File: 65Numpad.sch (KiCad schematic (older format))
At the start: 137 parts, among them J1 MX-NoLED, K1 MX-NoLED, M1 MX-NoLED, P1 MX-NoLED, Q1 MX-NoLED, T1 MX-NoLED, U1 ProMicro, U2 MX-NoLED, X1 MX-NoLED, Y1 MX-NoLED

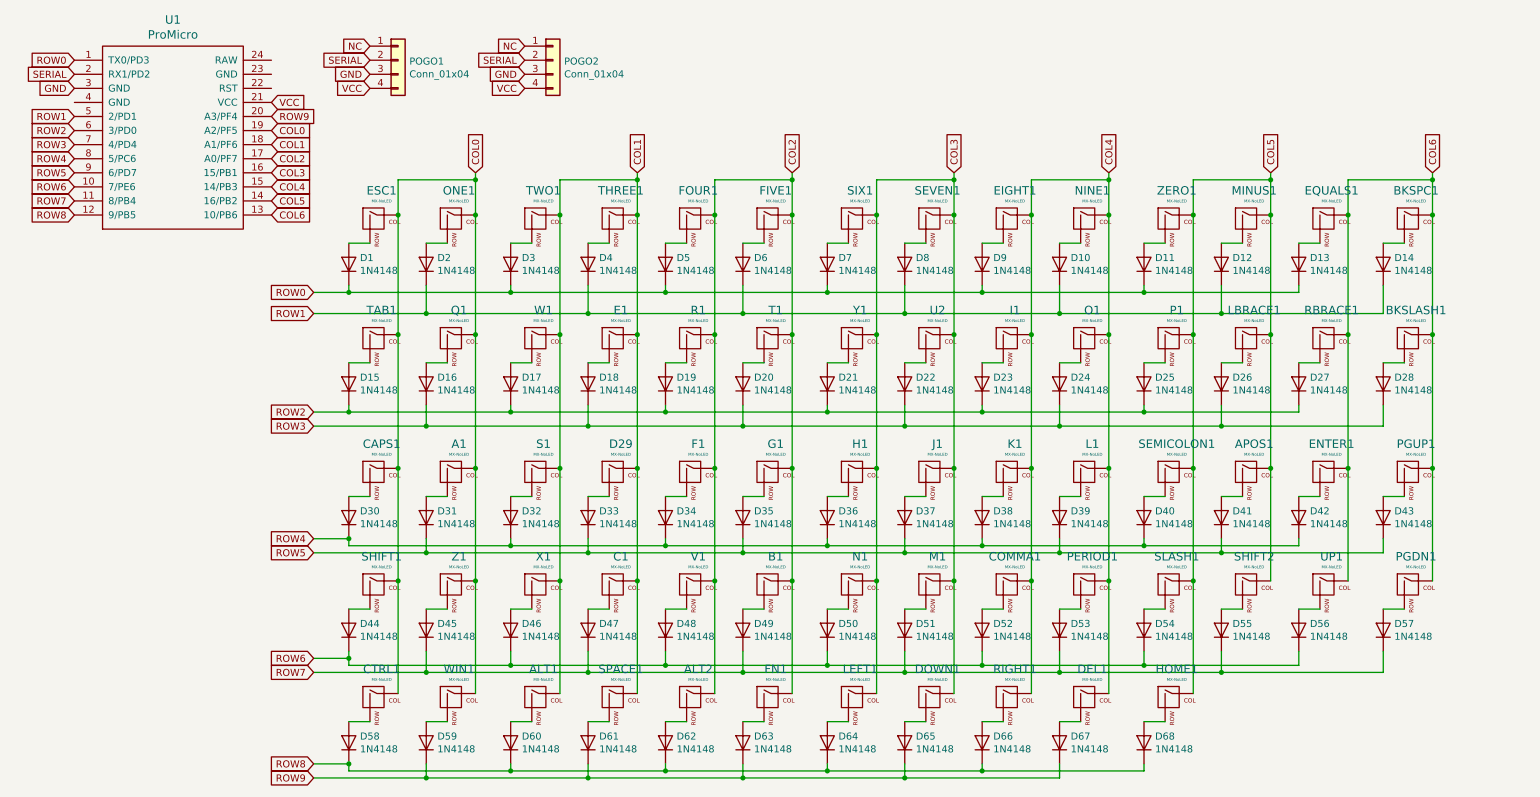
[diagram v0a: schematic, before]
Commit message: Arranged PCB
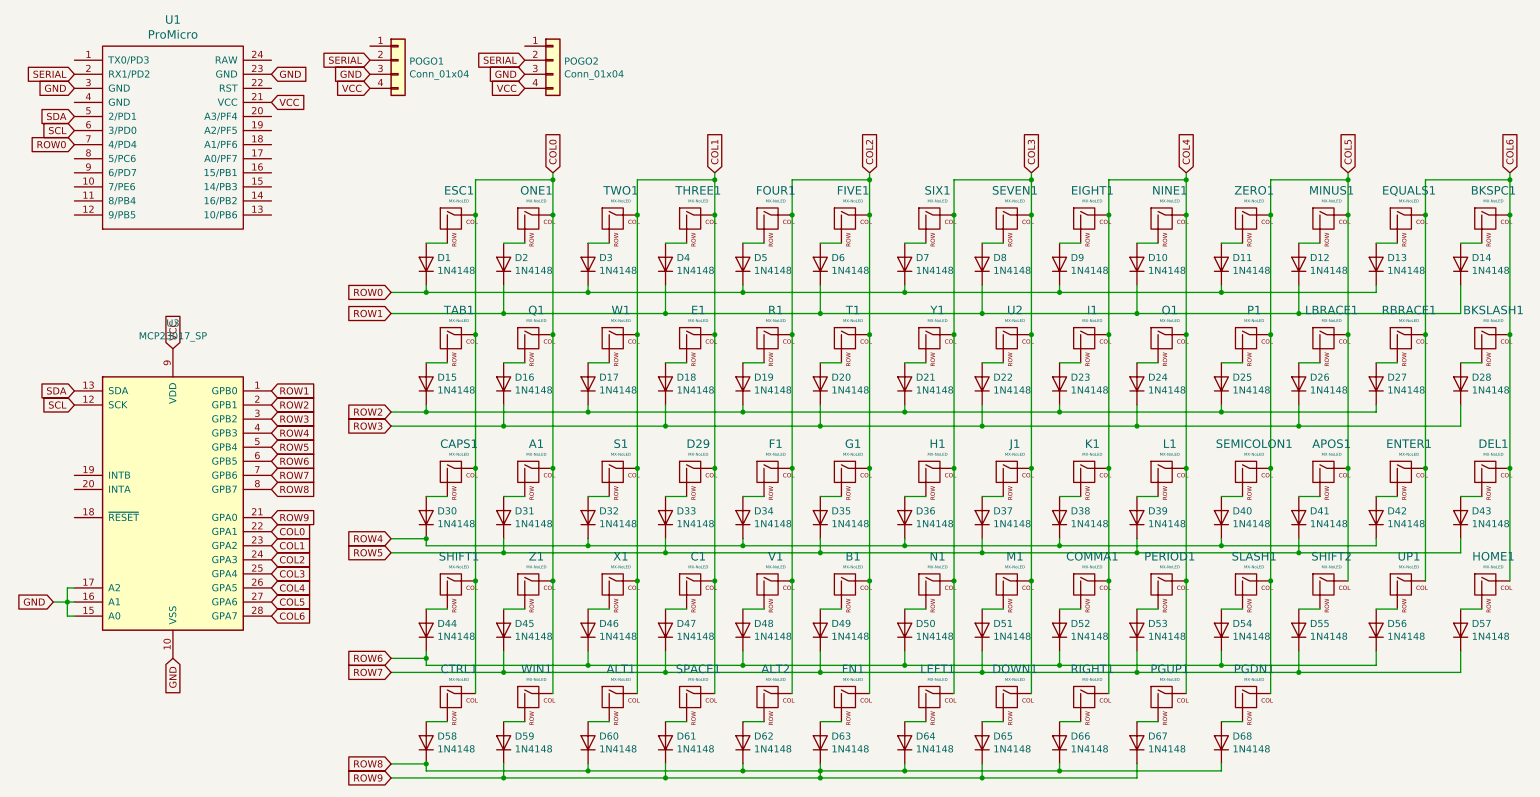
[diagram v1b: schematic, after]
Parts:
- added U3: MCP23017_SP, Package_DIP:DIP-28_W7.62mm, symbol Interface_Expansion:MCP23017_SP
- A1, APOS1, B1, C1, COMMA1, D29, DEL1, DOWN1, E1, EIGHT1, EQUALS1, ESC1, F1, FIVE1, FOUR1, G1, H1, HOME1, I1, J1, K1, L1, LBRACE1, LEFT1, M1, MINUS1, N1, NINE1, O1, ONE1, P1, PERIOD1, PGDN1, PGUP1, Q1, R1, RBRACE1, RIGHT1, S1, SEMICOLON1, SEVEN1, SIX1, SLASH1, T1, THREE1, TWO1, U2, UP1, V1, W1, X1, Y1, Z1, ZERO1: footprint MX_Only:MXOnly-1U-NoLED -> MX_Only:MXOnly-1U-NoLEDHotswap
- ALT1, ALT2, CTRL1, FN1, WIN1: footprint MX_Only:MXOnly-1.25U-NoLED -> MX_Only:MXOnly-1.25U-NoLEDHotswap
- BKSLASH1, TAB1: footprint MX_Only:MXOnly-1.5U-NoLED -> MX_Only:MXOnly-1.5U-NoLEDHotswap
- BKSPC1: footprint MX_Only:MXOnly-2U-NoLED -> MX_Only:MXOnly-2U-NoLEDHotswap
- CAPS1, SHIFT2: footprint MX_Only:MXOnly-1.75U-NoLED -> MX_Only:MXOnly-1.75U-NoLEDHotswap
- D1, D10, D11, D12, D13, D14, D15, D16, D17, D18, D19, D2, D20, D21, D22, D23, D24, D25, D26, D27, D28, D3, D30, D31, D32, D33, D34, D35, D36, D37, D38, D39, D4, D40, D41, D42, D43, D44, D45, D46, D47, D48, D49, D5, D50, D51, D52, D53, D54, D55, D56, D57, D58, D59, D6, D60, D61, D62, D63, D64, D65, D66, D67, D68, D7, D8, D9: footprint Diode_THT:D_DO-35_SOD27_P7.62mm_Horizontal -> Diodes_THT:D_DO-35_SOD27_P7.62mm_Horizontal
- ENTER1, SHIFT1: footprint MX_Only:MXOnly-2.25U-NoLED -> MX_Only:MXOnly-2.25U-NoLEDHotswap
- SPACE1: footprint MX_Only:MXOnly-6.25U-NoLED -> MX_Only:MXOnly-6.25U-NoLEDHotswap
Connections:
- net COL0: now also U3.22 (GPA1); no longer U1.19 (A2/PF5)
- net COL1: now also U3.23 (GPA2); no longer U1.18 (A1/PF6)
- net COL2: now also U3.24 (GPA3); no longer U1.17 (A0/PF7)
- net COL3: now also U3.25 (GPA4); no longer U1.16 (15/PB1)
- net COL4: now also PGUP1.1 (COL), U3.26 (GPA5); no longer DEL1.1 (COL), U1.15 (14/PB3)
- net COL5: now also PGDN1.1 (COL), U3.27 (GPA6); no longer HOME1.1 (COL), U1.14 (16/PB2)
- net COL6: now also DEL1.1 (COL), HOME1.1 (COL), U3.28 (GPA7); no longer PGDN1.1 (COL), PGUP1.1 (COL), U1.13 (10/PB6)
- net GND: now also U1.23 (GND), U3.10 (VSS), U3.15 (A0), U3.16 (A1), U3.17 (A2)
- net ROW0: now also U1.7 (4/PD4); no longer U1.1 (TX0/PD3)
- net ROW1: now also U3.1 (GPB0); no longer U1.5 (2/PD1)
- net ROW2: now also U3.2 (GPB1); no longer U1.6 (3/PD0)
- net ROW3: now also U3.3 (GPB2); no longer U1.7 (4/PD4)
- net ROW4: now also U3.4 (GPB3); no longer U1.8 (5/PC6)
- net ROW5: now also U3.5 (GPB4); no longer U1.9 (6/PD7)
- net ROW6: now also U3.6 (GPB5); no longer U1.10 (7/PE6)
- net ROW7: now also U3.7 (GPB6); no longer U1.11 (8/PB4)
- net ROW8: now also D59.1 (K), D61.1 (K), D63.1 (K), D65.1 (K), D67.1 (K), U3.21 (GPA0), U3.8 (GPB7); no longer U1.12 (9/PB5)
- net VCC: now also U3.9 (VDD)
- net at DEL1.2 (ROW): now also D43.2 (A); no longer D67.2 (A)
- net at HOME1.2 (ROW): now also D57.2 (A); no longer D68.2 (A)
- net at PGUP1.2 (ROW): now also D67.2 (A); no longer D43.2 (A)
- net at PGDN1.2 (ROW): now also D68.2 (A); no longer D57.2 (A)
- net NC: no longer names the net of POGO2.1 (Pin_1)
- net NC: no longer POGO1.1 (Pin_1)
- removed net ROW9: D59.1 (K), D61.1 (K), D63.1 (K), D65.1 (K), D67.1 (K), U1.20 (A3/PF4)
- new net SCL: U1.6 (3/PD0), U3.12 (SCK)
- new net SDA: U1.5 (2/PD1), U3.13 (SDA)
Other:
- moved on the sheet: A1, ALT1, ALT2, APOS1, B1, BKSLASH1, BKSPC1, C1, CAPS1, COMMA1, CTRL1, D1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

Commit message: Almost done routing
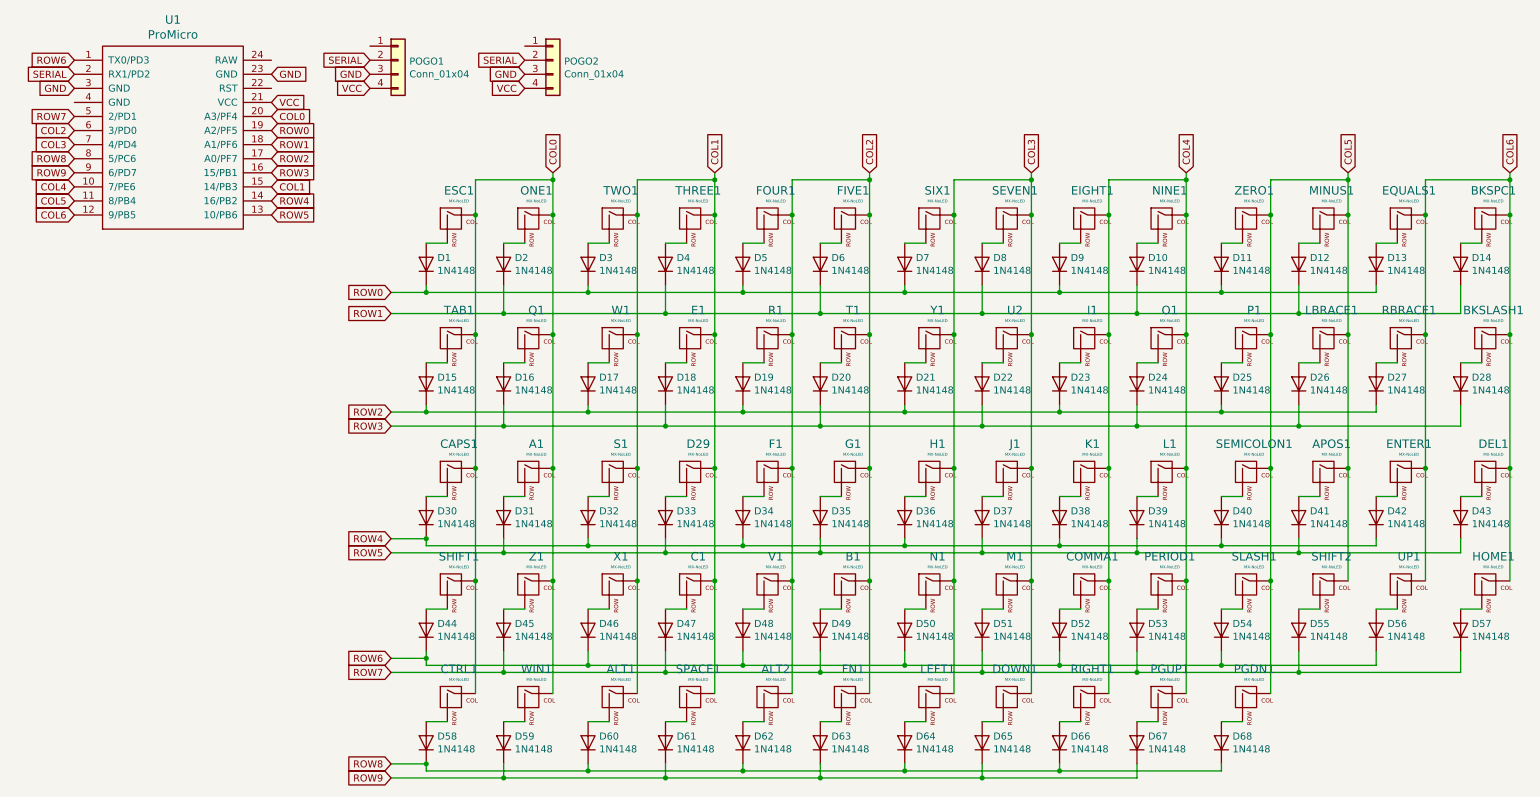
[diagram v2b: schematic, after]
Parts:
- removed U3: MCP23017_SP, Package_DIP:DIP-28_W7.62mm, symbol Interface_Expansion:MCP23017_SP
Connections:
- net SCL is gone; now on net COL2: U1.6 (3/PD0)
- net SDA is gone; now on net ROW7: U1.5 (2/PD1)
- net COL0: now also U1.20 (A3/PF4)
- net COL1: now also U1.15 (14/PB3)
- net COL3: now also U1.7 (4/PD4)
- net COL4: now also U1.10 (7/PE6)
- net COL5: now also U1.11 (8/PB4)
- net COL6: now also U1.12 (9/PB5)
- net ROW0: now also U1.19 (A2/PF5); no longer U1.7 (4/PD4)
- net ROW1: now also U1.18 (A1/PF6)
- net ROW2: now also U1.17 (A0/PF7)
- net ROW3: now also U1.16 (15/PB1)
- net ROW4: now also U1.14 (16/PB2)
- net ROW5: now also U1.13 (10/PB6)
- net ROW6: now also U1.1 (TX0/PD3)
- net ROW8: now also U1.8 (5/PC6); no longer D59.1 (K), D61.1 (K), D63.1 (K), D65.1 (K), D67.1 (K)
- net ROW9: now reaches U1.9 (6/PD7)
- net ROW9: now also D59.1 (K), D61.1 (K), D63.1 (K), D65.1 (K), D67.1 (K)
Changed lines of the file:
@@
 Connection ~ 3350 6000
-Wire Wire Line
-	6150 6050 6750 6050
 Wire Wire Line
 	3900 6000 3900 6100
@@
 	5600 6000 5600 6050
 Connection ~ 5600 6050
-Wire Wire Line
-	5600 6050 6150 6050
 Connection ~ 6150 6100
 Wire Wire Line
@@
 Text GLabel 4050 1100 0    50   Input ~ 0
 GND
-$Comp
-L Interface_Expansion:MCP23017_SP U3
-U 1 1 602098ED
-P 1550 4150
-F 0 "U3" H 1550 5431 50  0000 C CNN
-F 1 "MCP23017_SP" H 1550 5340 50  0000 C CNN
-F 2 "Package_DIP:DIP-28_W7.62mm" H 1750 3150 50  0001 L CNN
-F 3 "http://ww1.microchip.com/downloads/en/DeviceDoc/20001952C.pdf" H 1750 3050 50  0001 L CNN
-	1    1550 4150
-	1    0    0    -1
-$EndComp
-Connection ~ 6150 6050
 Wire Wire Line
 	6150 6050 6150 6100
-Text GLabel 1550 5250 3    50   Input ~ 0
-GND
-Text GLabel 1550 3050 1    50   Input ~ 0
-VCC
-Text GLabel 700  4850 0    50   Input ~ 0
-GND
 Text GLabel 2250 1100 2    50   Input ~ 0
 GND
+Text GLabel 2250 1400 2    50   Input ~ 0
+COL0
+Text GLabel 2250 1600 2    50   Input ~ 0
+ROW1
+Text GLabel 2250 1500 2    50   Input ~ 0
+ROW0
+Text GLabel 2250 1700 2    50   Input ~ 0
+ROW2
+Text GLabel 2250 1800 2    50   Input ~ 0
+ROW3
+Text GLabel 2250 1900 2    50   Input ~ 0
+COL1
+Text GLabel 2250 2100 2    50   Input ~ 0
+ROW5
+Text GLabel 2250 2000 2    50   Input ~ 0
+ROW4
+Text GLabel 850  1500 0    50   Input ~ 0
+COL2
+Text GLabel 850  1000 0    50   Input ~ 0
+ROW6
 Text GLabel 850  1400 0    50   Input ~ 0
-SDA
-Text GLabel 850  1500 0    50   Input ~ 0
-SCL
-Text GLabel 850  3350 0    50   Input ~ 0
-SDA
-Text GLabel 850  3450 0    50   Input ~ 0
-SCL
+ROW7
+Text GLabel 850  1600 0    50   Input ~ 0
+COL3
 Wire Wire Line
-	850  4950 800  4950
-Wire Wire Line
-	800  4950 800  4850
-Wire Wire Line
-	800  4850 700  4850
-Wire Wire Line
-	800  4850 850  4850
-Connection ~ 800  4850
-Wire Wire Line
-	800  4850 800  4750
-Wire Wire Line
-	800  4750 850  4750
-Text GLabel 2250 4950 2    50   Input ~ 0
+	5600 6050 6750 6050
+Text GLabel 850  1700 0    50   Input ~ 0
+ROW8
+Text GLabel 850  1800 0    50   Input ~ 0
+ROW9
+Text GLabel 850  1900 0    50   Input ~ 0
+COL4
+Text GLabel 850  2000 0    50   Input ~ 0
+COL5
+Text GLabel 850  2100 0    50   Input ~ 0
 COL6
-Text GLabel 2250 4850 2    50   Input ~ 0
-COL5
-Text GLabel 2250 4750 2    50   Input ~ 0
-COL4
-Text GLabel 2250 4650 2    50   Input ~ 0
-COL3
-Text GLabel 2250 4550 2    50   Input ~ 0
-COL2
-Text GLabel 2250 4450 2    50   Input ~ 0
-COL1
-Text GLabel 2250 4350 2    50   Input ~ 0
-COL0
-Text GLabel 2250 4250 2    50   Input ~ 0
-ROW9
-Text GLabel 2250 4050 2    50   Input ~ 0
-ROW8
-Text GLabel 2250 3950 2    50   Input ~ 0
-ROW7
-Text GLabel 2250 3850 2    50   Input ~ 0
-ROW6
-Text GLabel 2250 3750 2    50   Input ~ 0
-ROW5
-Text GLabel 2250 3550 2    50   Input ~ 0
-ROW3
-Text GLabel 2250 3650 2    50   Input ~ 0
-ROW4
-Text GLabel 2250 3450 2    50   Input ~ 0
-ROW2
-Text GLabel 2250 3350 2    50   Input ~ 0
-ROW1
-Text GLabel 850  1600 0    50   Input ~ 0
-ROW0
 $EndSCHEMATC
